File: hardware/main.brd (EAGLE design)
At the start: 60.9 x 38.1 mm, 35 parts, among them IC1 LM358D, IC2 MC34063, T3 IRF840

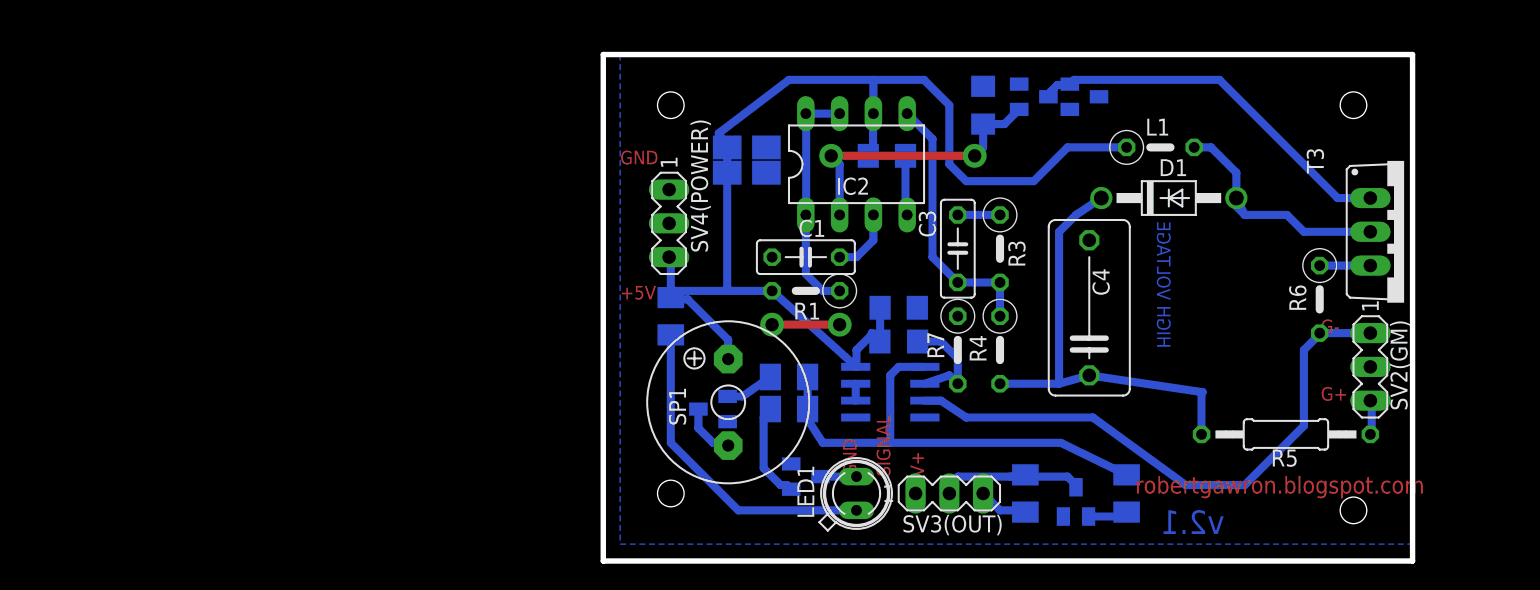
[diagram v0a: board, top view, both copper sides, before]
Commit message: PCB is now fixed.
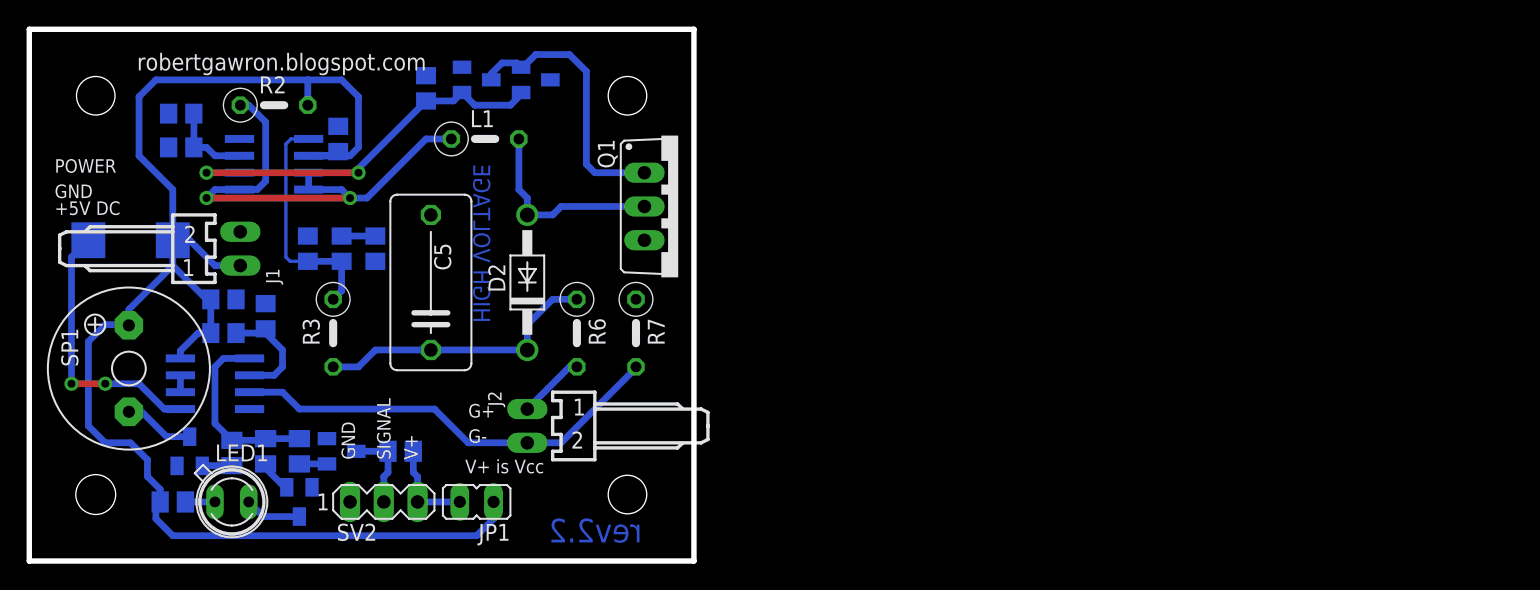
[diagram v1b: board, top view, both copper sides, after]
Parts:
- removed IC1: LM358D, linear:SO08
- removed SV2(GM), SV3(OUT), SV4(POWER): (no value), con-lstb:MA03-1
- removed T2, T6, T7: (no value), transistor-npn:SOT23
- removed T3: IRF840, transistor-power:TO220BV
- added IC3: MC34063AD, mc34063:SOIC8
- added J1, J2: 22-05-7028-02, con-molex:7395-02
- added JP1: (no value), jumper:JP1
- added Q1: IRF840, transistor-power:TO220BV
- added Q2, Q3, Q4: (no value), transistor-npn:SOT23
- added R14: (no value), resistor:M0805
- added SV2: (no value), con-lstb:MA03-1
- C1: device resistor:C050-025X075 -> resistor:C0805
- C2: value 100n -> 32n; device resistor:C3216 -> resistor:C0805
- C3: value 10n -> 100n; device resistor:C050-025X075 -> resistor:C0805
- C4: value 100n/630V -> 10n; device resistor:C102-064X133 -> resistor:C0805
- C5: value 100n -> 100n/630V; device resistor:C3216 -> resistor:C102-064X133
- C6: value 330u -> 100n; device resistor:A/3216-18W -> resistor:C0805
- C7: device resistor:A/3216-18W -> rcl:D/7343-31R
- D1: value 1n4007 -> BAS40; device diode:DO41-10 -> diode:SOT23
- D2: value BAS40 -> 1n4007; device diode:SOT23 -> diode:DO41-10
- IC2: value MC34063 -> LM358D; device ic-package:DIL08 -> linear:SO08
- R1: value R22/0.5W -> 10k; device resistor:0207/5V -> resistor:R0805
- R10, R11: device resistor:M1206 -> resistor:M0805
- R12: value 510R -> 1k; device resistor:M1206 -> resistor:M0805
- R13: value (none) -> 510R; device resistor:M1206 -> resistor:M0805
- R2: value 10k -> R22/0.5W; device resistor:R1206 -> resistor:0207/5V
- R3: value 30k+1k -> 10M
- R4: value 10M -> 30k+1k; device resistor:0207/5V -> resistor:R0805
- R5: value 6M8 -> 30k+1k; device resistor:0207/12 -> resistor:R0805
- R6: value 10k -> 6M8
- R7: value 470R -> 10k
- R8: device resistor:R1206 -> resistor:R0805
- R9: value 1k -> 470R; device resistor:M1206 -> resistor:R0805
- moved R5 69.9 mm to (26.0, 23.5), flipped to the bottom, turned to 90 degrees
- moved R9 66.1 mm to (17.8, 18.4)
- moved R13 64.1 mm to (10.8, 4.45), turned to 0 degrees
- moved C4 59.0 mm to (21.0, 23.5), flipped to the bottom
- moved R6 55.9 mm to (41.2, 17.1)
- moved R2 53.3 mm to (18.4, 34.3), flipped to the top, turned to 0 degrees
- moved C2 53.1 mm to (11.4, 31.1), turned to 0 degrees
- moved D1 52.8 mm to (33.7, 36.2), flipped to the bottom, turned to 90 degrees
- moved IC2 51.0 mm to (14.0, 13.3), flipped to the bottom, turned to 270 degrees
- moved L1 50.8 mm to (34.3, 31.8)
- moved R8 50.8 mm to (14.6, 17.1)
- moved R3 50.6 mm to (22.9, 17.1)
- moved R4 50.1 mm to (23.5, 23.5), flipped to the bottom
- moved C1 48.2 mm to (11.4, 33.7), flipped to the bottom, turned to 0 degrees
- moved C3 47.3 mm to (23.2, 31.8), flipped to the bottom
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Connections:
- removed net N$20: R5.2, SV2(GM).3
- new net N$18: J2.1, R6.2
- new net N$7: IC3.1, IC3.7, IC3.8, L1.1, R2.1
- net N$1: now also Q4.1, R12.2; no longer R9.2, T7.1
- net N$10: now also Q2.1, R10.2; no longer R11.2, T2.1
- net N$11: now also R4.1, R5.2; no longer IC2.1, IC2.7, IC2.8, R1.1
- net N$12: now also C5.1, D2.C, R3.2, R6.1; no longer C4.1, D1.C, R4.2, R5.1
- net N$13: now also C4.1, IC3.5, R3.1, R4.2; no longer C3.1, IC2.5, R3.2, R4.1
- net N$14: now also D1.1, IC3.2, R1.2; no longer D2.1, IC2.2, R2.2
- net N$15: now also D2.A, Q1.D; no longer D1.A, T3.D
- net N$16: now also D1.3, Q1.G; no longer D2.3, T3.G
- net N$17: now also IC2.3, J2.2, R7.2; no longer IC1.3, R6.2, SV2(GM).1
- net N$19: now also IC2.2, R9.2; no longer IC1.2, R7.2
- net N$2: now also Q3.1, R11.2; no longer R10.2, T6.1
- net N$21: now also JP1.2, R14.2, SV2.3; no longer R13.2, SV3(OUT).3
- net N$22: now also IC2.6, IC2.7; no longer IC1.6, IC1.7
- net N$3: now also Q3.3; no longer T6.3
- net N$4: now also Q4.3, R14.1, SV2.2; no longer R13.1, SV3(OUT).2, T7.3
- net N$5: now also C2.1, IC3.3; no longer IC2.3
- net N$6: now also R13.1; no longer R12.1
- net N$8: now also IC2.1, R12.1; no longer IC1.1, R9.1
- net N$9: now also Q2.3; no longer T2.3
- net V+: now also C3.1, C6.1, IC2.8, IC3.6, J1.1, JP1.1, R13.2, R2.2; no longer C2.1, C5.1, C6.+, IC1.8, IC2.6, L1.1, R1.2, R12.2, SV4(POWER).3
- net V-: now also C6.2, IC2.5, IC3.4, J1.2, Q1.S, Q2.2, Q3.2, Q4.2, R1.1, R5.1, R9.1, SV2.1; no longer C6.-, IC1.4, IC1.5, R2.1, R3.1, R6.1, SV3(OUT).1, SV4(POWER).1, T2.2, T3.S, T6.2, T7.2
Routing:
- net N$7: track 0.00 -> 36.8 mm, vias 0 -> 2
- net N$8: track 36.8 -> 14.0 mm
- net V+: track 90.8 -> 113.1 mm
- net N$6: track 24.2 -> 2.23 mm
- net N$11: track 17.7 -> 2.54 mm
- net N$12: track 34.1 -> 21.6 mm
- net N$17: track 43.7 -> 33.1 mm
- net N$14: track 21.3 -> 30.2 mm
- net N$16: track 28.7 -> 20.6 mm
- net N$18: track 0.00 -> 5.13 mm
- net N$2: track 7.39 -> 2.51 mm
- net N$4: track 11.0 -> 6.34 mm
- net V-: track 16.6 -> 20.3 mm
- net N$21: track 3.75 -> 7.12 mm
- net N$15: track 18.2 -> 15.1 mm
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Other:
- board size 60.9 x 38.1 mm -> 50 x 40 mm
- board text added: "+5V DC"
- board text added: "POWER"
- board text added: "V+ is Vcc"
- board text added: "rev2.2"
- board text removed: "+5V"
- board text removed: "v2.1"
